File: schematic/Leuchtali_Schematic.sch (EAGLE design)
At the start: 17 parts, among them IC4 LT1618EMS#PBF

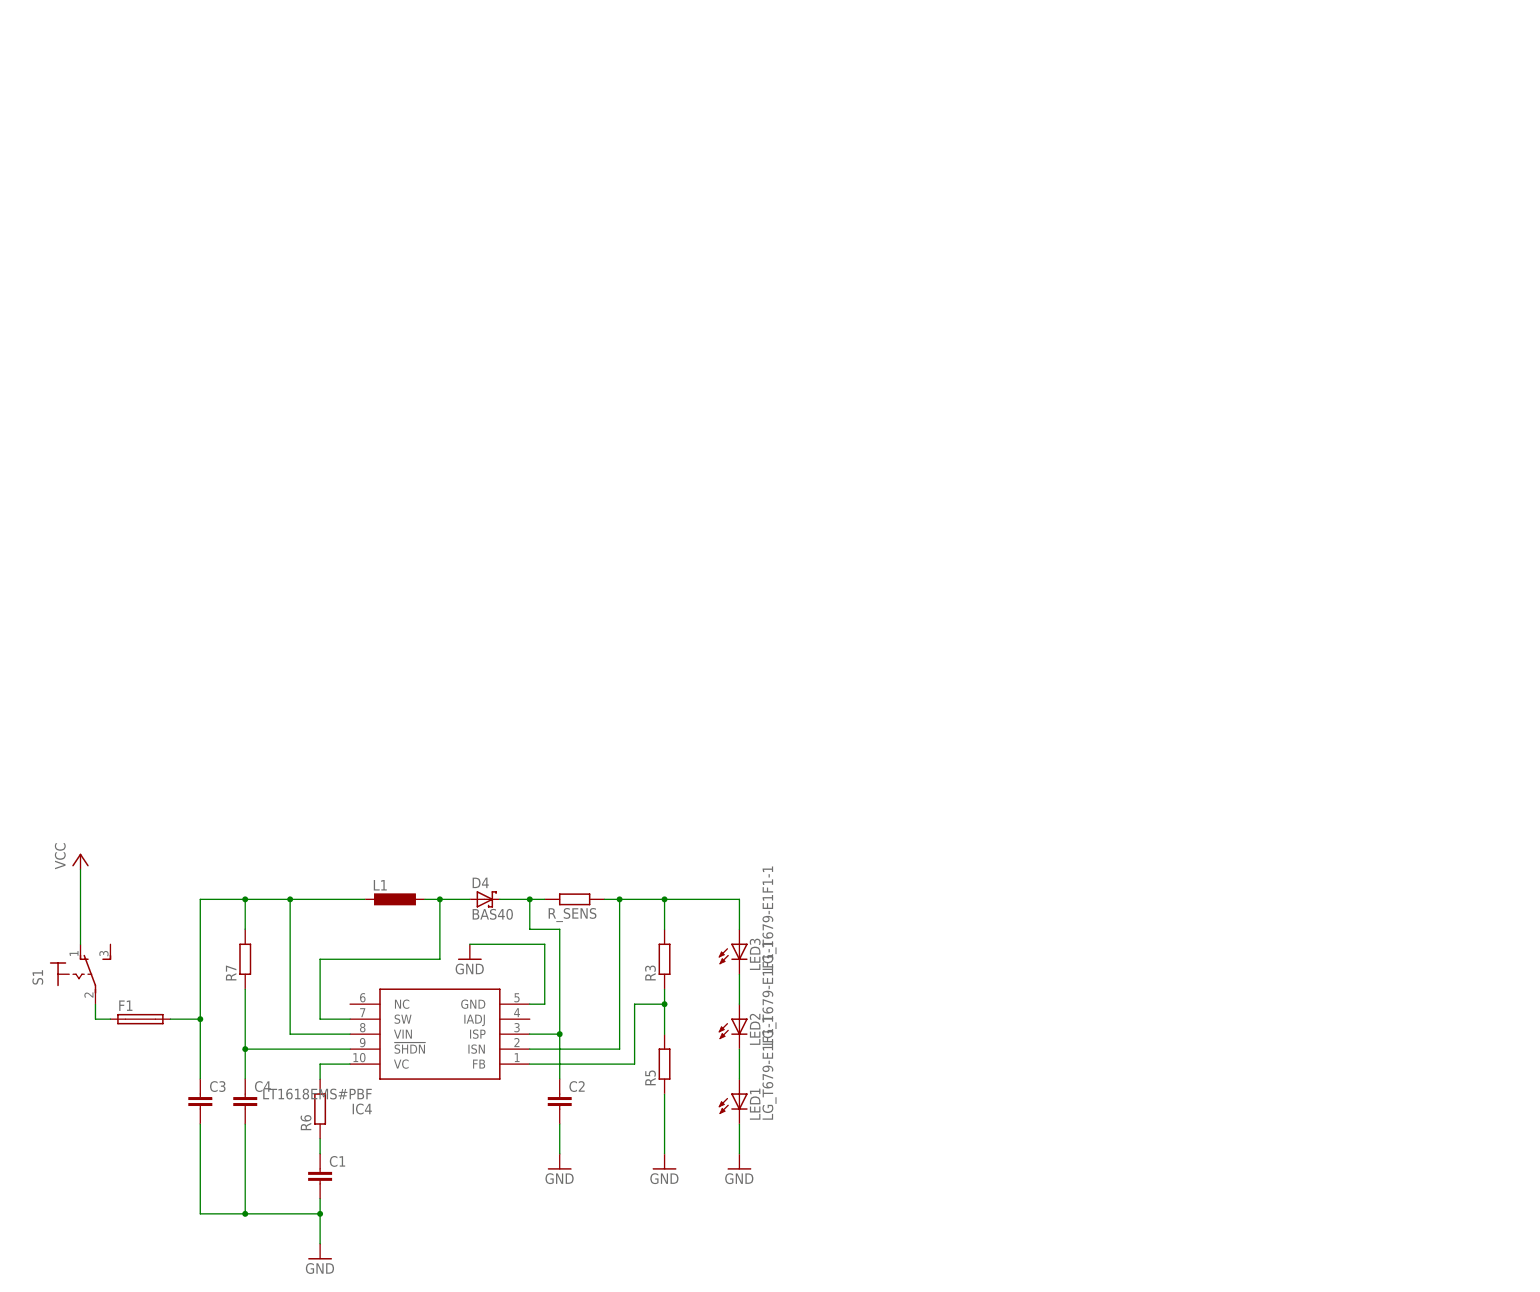
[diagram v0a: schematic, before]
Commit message: Continued working on the schematic
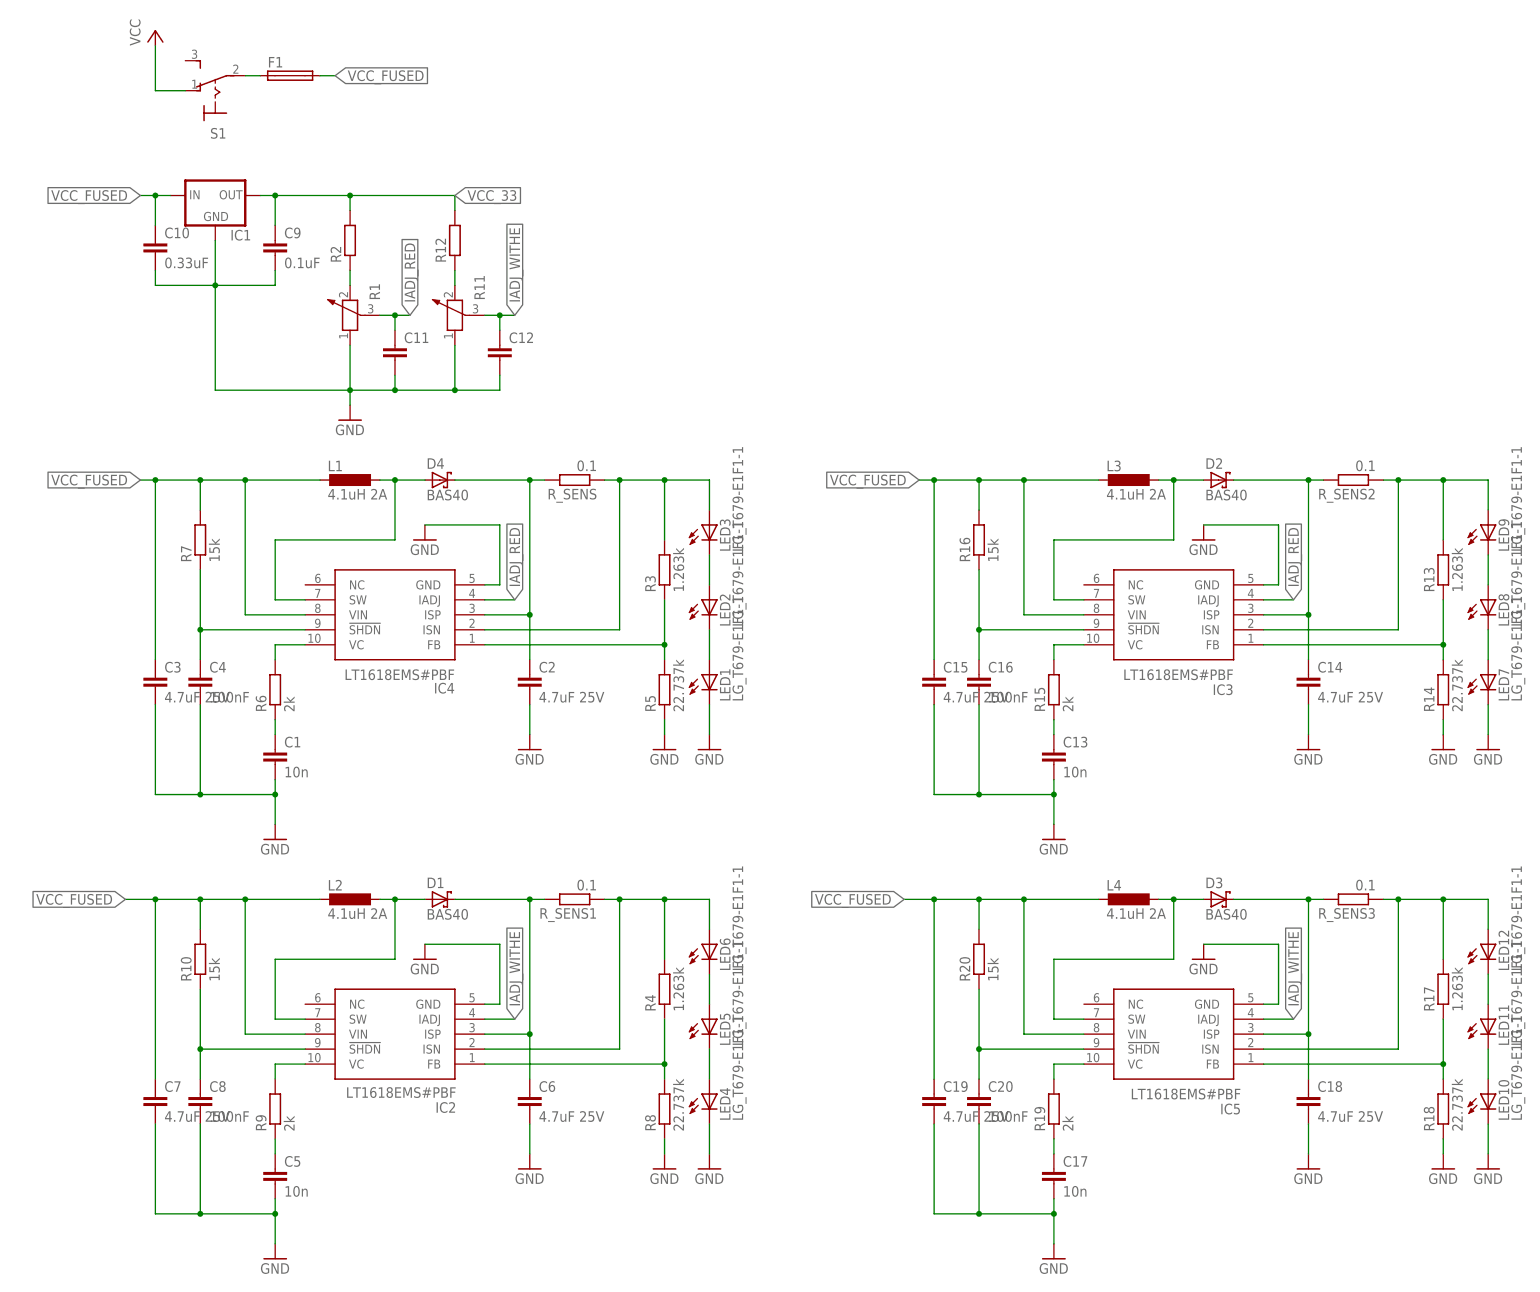
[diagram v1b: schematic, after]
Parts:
- added C10: 0.33uF, rcl:C-EU025-024X044
- added C11, C12: (no value), rcl:C-EU025-024X044
- added C13, C17, C5: 10n, rcl:C-EUC0805
- added C14, C15, C18, C19, C6, C7: 4.7uF 25V, rcl:C-EUC0805
- added C16, C20, C8: 100nF, rcl:C-EUC0805
- added C9: 0.1uF, rcl:C-EU025-024X044
- added D1, D2, D3: BAS40, diode:BAS40
- added IC1: (no value), v-reg:78LXX
- added IC2, IC3, IC5: LT1618EMS#PBF, LT1618EMS:LT1618EMS#PBF
- added L2, L3, L4: 4.1uH 2A, rcl:L-EU0204/5
- added LED10, LED11, LED12, LED4, LED5, LED6, LED7, LED8, LED9: LG_T679-E1F1-1, led:LG_T679-E1F1-1
- added R1, R11: (no value), rcl:POTENTIOMETER_PT-10
- added R10, R16, R20: 15k, rcl:R-EU_R0805
- added R12, R2: (no value), rcl:R-EU_R0805
- added R13, R17, R4: 1.263k, rcl:R-EU_R0805
- added R14, R18, R8: 22.737k, rcl:R-EU_R0805
- added R15, R19, R9: 2k, rcl:R-EU_R0805
- added R_SENS1, R_SENS2, R_SENS3: 0.1, rcl:R-EU_R0805
- C1: value (none) -> 10n
- C2, C3: value (none) -> 4.7uF 25V
- C4: value (none) -> 100nF
- L1: value (none) -> 4.1uH 2A
- R3: value (none) -> 1.263k
- R5: value (none) -> 22.737k
- R6: value (none) -> 2k
- R7: value (none) -> 15k
- R_SENS: value (none) -> 0.1
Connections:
- new net IADJ_RED: C11.1, IC3.IADJ, IC4.IADJ, R1.3
- new net IADJ_WITHE: C12.1, IC2.IADJ, IC5.IADJ, R11.3
- new net N$1: R11.2, R12.1
- new net N$10: IC2.FB, R4.1, R8.2
- new net N$11: IC2.VC, R9.2
- new net N$12: C5.1, R9.1
- new net N$2: LED7.A, LED8.C
- new net N$23: C8.1, IC2.!SHDN, R10.1
- new net N$25: C14.1, D2.C, IC3.ISP, R_SENS2.2
- new net N$26: IC3.ISN, LED9.A, R13.2, R_SENS2.1
- new net N$27: IC3.FB, R13.1, R14.2
- new net N$28: IC3.VC, R15.2
- new net N$29: C13.1, R15.1
- new net N$3: R1.2, R2.1
- new net N$30: C16.1, IC3.!SHDN, R16.1
- new net N$31: LED10.A, LED11.C
- new net N$32: LED11.A, LED12.C
- new net N$33: D3.A, IC5.SW, L4.1
- new net N$34: C18.1, D3.C, IC5.ISP, R_SENS3.2
- new net N$35: IC5.ISN, LED12.A, R17.2, R_SENS3.1
- new net N$36: IC5.FB, R17.1, R18.2
- new net N$37: IC5.VC, R19.2
- new net N$38: C17.1, R19.1
- new net N$39: C20.1, IC5.!SHDN, R20.1
- new net N$4: LED8.A, LED9.C
- new net N$5: LED4.A, LED5.C
- new net N$6: LED5.A, LED6.C
- new net N$7: D1.A, IC2.SW, L2.1
- new net N$8: C6.1, D1.C, IC2.ISP, R_SENS1.2
- new net N$9: IC2.ISN, LED6.A, R4.2, R_SENS1.1
- new net VCC_33: C9.1, IC1.OUT, R12.2, R2.2
- new net VCC_FUSED: C10.1, C15.1, C19.1, C3.1, C7.1, F1.2, IC1.IN, IC2.VIN, IC3.VIN, IC4.VIN, IC5.VIN, L1.2, L2.2, L3.2, L4.2, R10.2, R16.2, R20.2, R7.2
- net GND: now also C10.2, C11.2, C12.2, C13.2, C14.2, C15.2, C16.2, C17.2, C18.2, C19.2, C20.2, C5.2, C6.2, C7.2, C8.2, C9.2, IC1.GND, IC2.GND, IC3.GND, IC5.GND, LED10.C, LED4.C, LED7.C, R1.1, R11.1, R14.1, R18.1, R8.1
- net N$22: now also D2.A, IC3.SW, L3.1; no longer C3.1, F1.2, IC4.VIN, L1.2, R7.2
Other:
- moved on the sheet: C1, C2, C3, C4, D4, F1, IC4, L1, LED1, LED2, LED3, R3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
